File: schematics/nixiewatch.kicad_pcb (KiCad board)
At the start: 2 copper layers, 70 x 50 mm, 21 parts, among them Q1 BC546, Q2 6N90C, U1 NE555P

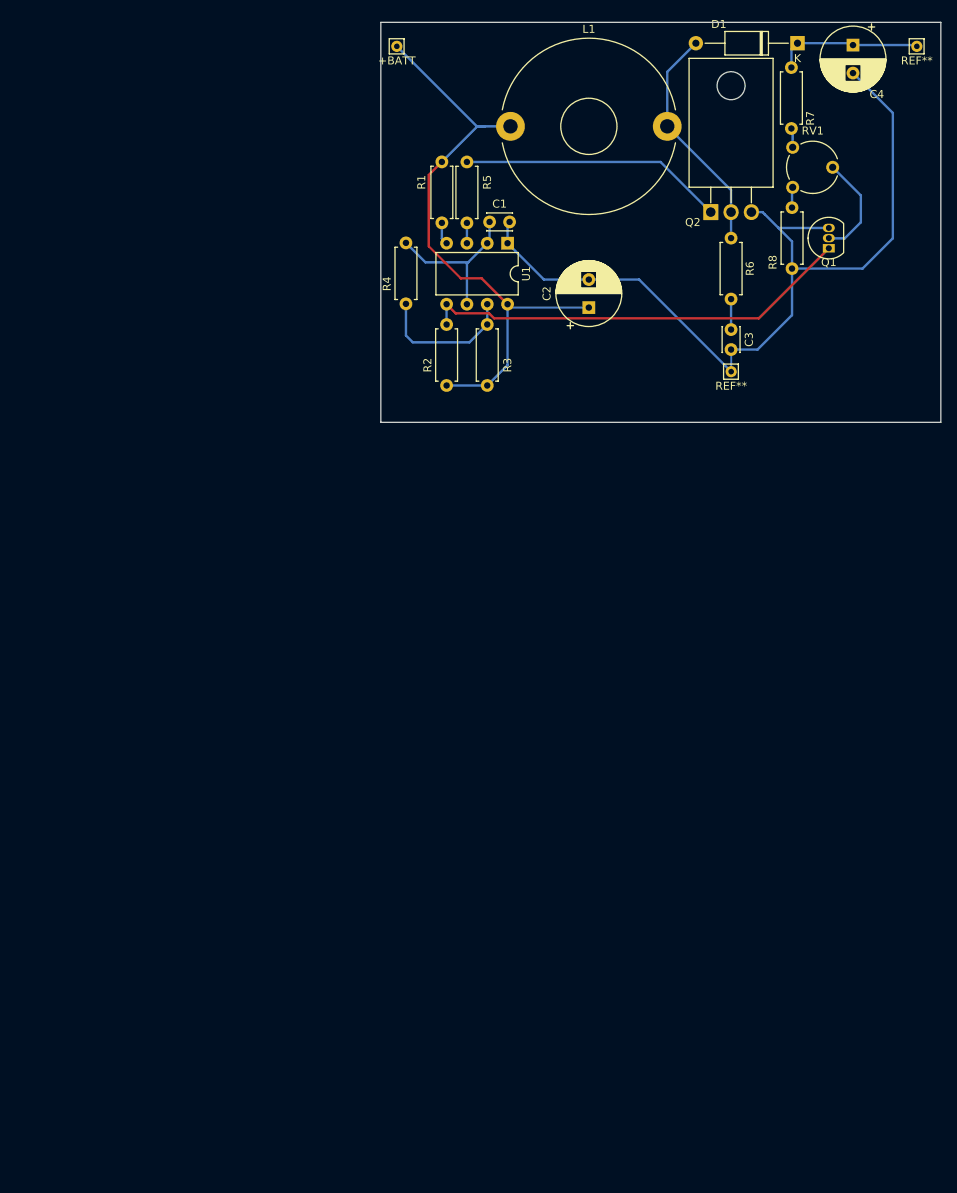
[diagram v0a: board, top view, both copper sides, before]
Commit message: pcb layout
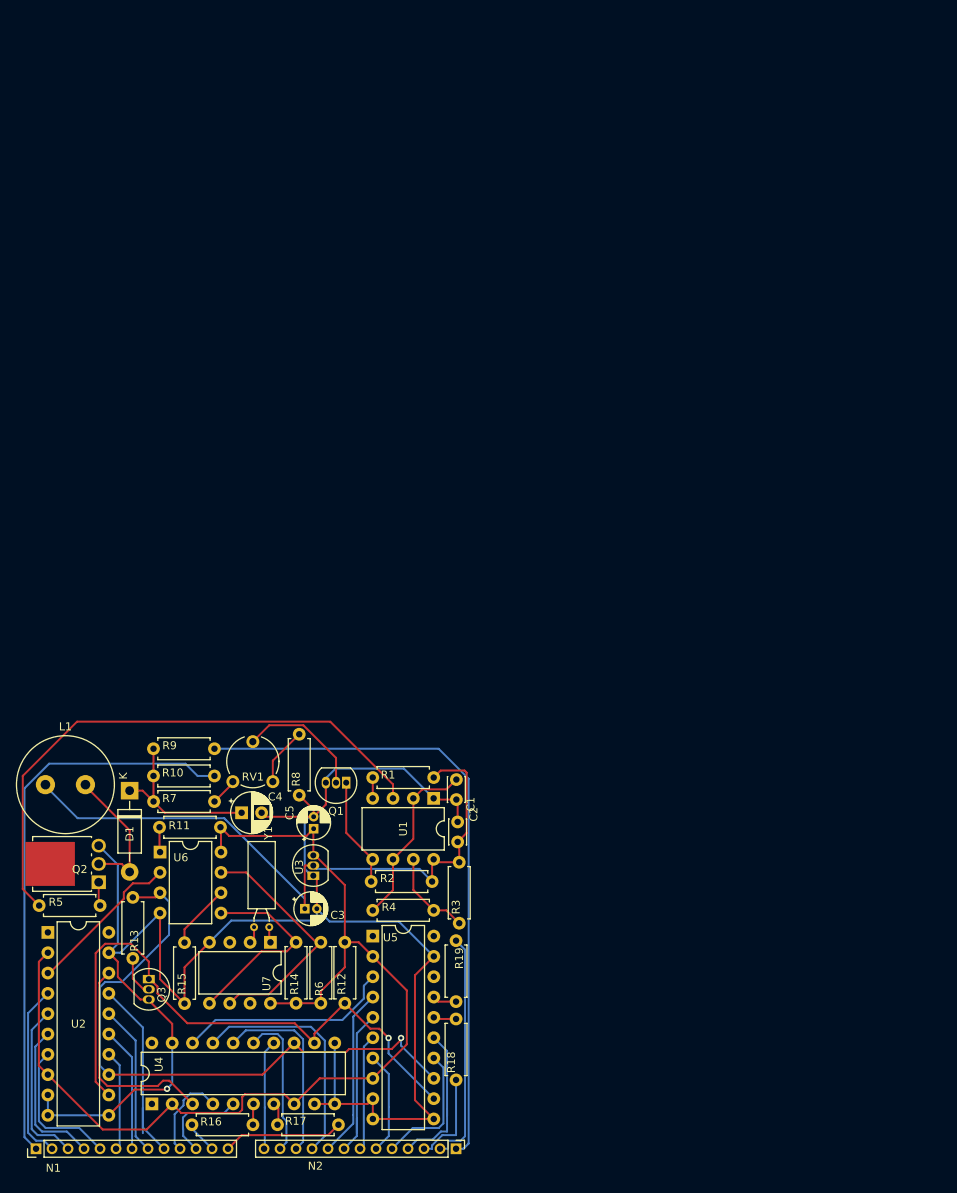
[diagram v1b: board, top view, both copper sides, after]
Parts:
- removed +BATT: +8V, Connector_Pin:Pin_D0.7mm_L6.5mm_W1.8mm_FlatFork
- removed REF**: GND, Connector_Pin:Pin_D0.7mm_L6.5mm_W1.8mm_FlatFork
- removed REF**: +170V, Connector_Pin:Pin_D0.7mm_L6.5mm_W1.8mm_FlatFork
- added C5: 33u, Capacitor_THT:CP_Radial_D4.0mm_P1.50mm, F.Cu at (83.6, 129.8)
- added N1: IN-16, Connector_PinHeader_2.00mm:PinHeader_1x13_P2.00mm_Vertical, F.Cu at (48.9, 169.8)
- added N2: IN-16, Connector_PinHeader_2.00mm:PinHeader_1x13_P2.00mm_Vertical, F.Cu at (101.4, 169.8)
- added Q3: BC546, Package_TO_SOT_THT:TO-92_Inline, F.Cu at (63.0, 148.6)
- added R10: 20k, Resistor_THT:R_Axial_DIN0207_L6.3mm_D2.5mm_P7.62mm_Horizontal, F.Cu at (71.2, 123.2)
- added R11: 20k, Resistor_THT:R_Axial_DIN0207_L6.3mm_D2.5mm_P7.62mm_Horizontal, F.Cu at (64.3, 129.6)
- added R12: 47k, Resistor_THT:R_Axial_DIN0207_L6.3mm_D2.5mm_P7.62mm_Horizontal, F.Cu at (87.5, 151.6)
- added R13: 6k8, Resistor_THT:R_Axial_DIN0207_L6.3mm_D2.5mm_P7.62mm_Horizontal, F.Cu at (61.0, 146.0)
- added R14: 2k2, Resistor_THT:R_Axial_DIN0207_L6.3mm_D2.5mm_P7.62mm_Horizontal, F.Cu at (81.4, 151.6)
- added R15: 20k, Resistor_THT:R_Axial_DIN0207_L6.3mm_D2.5mm_P7.62mm_Horizontal, F.Cu at (67.5, 151.7)
- added R16: 100k, Resistor_THT:R_Axial_DIN0207_L6.3mm_D2.5mm_P7.62mm_Horizontal, F.Cu at (68.4, 166.8)
- added R17: 100k, Resistor_THT:R_Axial_DIN0207_L6.3mm_D2.5mm_P7.62mm_Horizontal, F.Cu at (86.7, 166.8)
- added R18: 100k, Resistor_THT:R_Axial_DIN0207_L6.3mm_D2.5mm_P7.62mm_Horizontal, F.Cu at (101.4, 161.2)
- added R19: 100k, Resistor_THT:R_Axial_DIN0207_L6.3mm_D2.5mm_P7.62mm_Horizontal, F.Cu at (101.4, 143.8)
- added R9: 20k, Resistor_THT:R_Axial_DIN0207_L6.3mm_D2.5mm_P7.62mm_Horizontal, F.Cu at (71.2, 119.8)
- added U2: TPIC6B595, Package_DIP:DIP-20_W7.62mm, F.Cu at (50.4, 142.8)
- added U3: 5V MCP1702, Package_TO_SOT_THT:TO-92_Inline, F.Cu at (83.6, 135.7)
- added U4: TPIC6B595, Package_DIP:DIP-20_W7.62mm, F.Cu at (63.4, 164.2)
- added U5: TPIC6B595, Package_DIP:DIP-20_W7.62mm, F.Cu at (91.0, 143.2)
- added U6: ATtiny45V-10P, Package_DIP:DIP-8_W7.62mm, F.Cu at (64.4, 132.7)
- added U7: DS1307+, Package_DIP:DIP-8_W7.62mm, F.Cu at (78.2, 144.0)
- added Y1: 32.768kHz 12.5pF, Crystal:Crystal_C38-LF_D3.0mm_L8.0mm_Horizontal, F.Cu at (78.0, 142.1)
- C2: value 330u -> 100n; footprint Capacitor_THT:CP_Radial_D8.0mm_P3.50mm -> Capacitor_THT:C_Disc_D3.0mm_W2.0mm_P2.50mm
- C3: value 100p -> 33u; footprint Capacitor_THT:C_Disc_D3.0mm_W2.0mm_P2.50mm -> Capacitor_THT:CP_Radial_D4.0mm_P1.50mm
- C4: value 4u7 400V -> 1u 200V; footprint Capacitor_THT:CP_Radial_D8.0mm_P3.50mm -> Capacitor_THT:CP_Radial_D5.0mm_P2.50mm
- D1: value 200V -> 1N4007; footprint Diode_THT:D_A-405_P12.70mm_Horizontal -> Diode_THT:D_DO-41_SOD81_P10.16mm_Horizontal
- L1: value 287u -> 180u; footprint Inductor_THT:L_Toroid_Horizontal_D21.8mm_P19.60mm_Bourns_2100 -> Inductor_THT:L_Radial_D12.0mm_P5.00mm_Neosid_SD12k_style2
- Q2: value 6N90C -> IPU80R1K0CE; footprint Package_TO_SOT_THT:TO-220F-3_Horizontal_TabDown -> Package_TO_SOT_THT:SIPAK-1EP_Horizontal_TabDown
- R7: value 640k -> 680k
- moved D1 125.3 mm to (60.6, 125.0), turned to -90 degrees
- moved C4 122.7 mm to (74.6, 127.8), turned to 0 degrees
- moved R7 121.6 mm to (63.6, 126.4), turned to 0 degrees
- moved Q2 113.4 mm to (56.7, 136.5), turned to 90 degrees
- moved R6 108.5 mm to (84.5, 151.6), turned to 90 degrees
- moved R5 103.6 mm to (56.9, 139.4), turned to 180 degrees
- moved L1 100.8 mm to (50.1, 124.3)
- moved RV1 98.7 mm to (78.5, 123.9), turned to 90 degrees
- moved R8 90.2 mm to (81.8, 118.0)
- moved Q1 90.0 mm to (87.7, 124.0), turned to 180 degrees
- moved C3 89.9 mm to (82.5, 139.8), turned to 0 degrees
- moved R1 77.0 mm to (98.6, 123.4), turned to 180 degrees
- moved R4 75.9 mm to (98.6, 140.0), turned to 180 degrees
- moved U1 70.0 mm to (98.6, 126.0)
- moved C1 69.8 mm to (101.4, 123.7), turned to -90 degrees
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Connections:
- C3 pad 1: Net-(C3-Pad1) -> +BATT
- R6 pad 1: Net-(D1-A) -> Net-(U2-VCC)
- R6 pad 2: Net-(C3-Pad1) -> Net-(U6-PB2)
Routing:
- net Net-(U2-VCC): track 0.00 -> 135.5 mm
- net GND: track 108.5 -> 216.1 mm, vias 0 -> 1
- net Net-(N2-PadA): track 0.00 -> 80.8 mm
- net Net-(U2-SRCK): track 0.00 -> 78.3 mm, vias 0 -> 1
- net Net-(Q3-C): track 0.00 -> 76.9 mm, vias 0 -> 1
- net Net-(N1-PadA): track 0.00 -> 71.3 mm
- net Net-(U1-OUT): track 2.54 -> 71.8 mm
- net Net-(Q1-C): track 54.7 -> 13.8 mm
- net Net-(U6-PB2): track 0.00 -> 30.6 mm
- net Net-(Q2-G): track 33.1 -> 2.99 mm
- net Net-(U4-DRAIN7): track 0.00 -> 29.7 mm
- net Net-(N2-PadRHDP): track 0.00 -> 29.3 mm
- net Net-(U2-SER_OUT): track 0.00 -> 27.2 mm
- net Net-(U4-SER_OUT): track 0.00 -> 26.9 mm
- net Net-(U2-DRAIN7): track 0.00 -> 25.4 mm
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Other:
- board outline removed
